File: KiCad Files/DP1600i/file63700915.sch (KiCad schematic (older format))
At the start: 22 parts, among them J1 DB25_Male, J11 Conn_01x05, J12 Conn_01x05, J13 Conn_01x05, J14 Conn_01x05, J15 Conn_01x05, J16 Conn_01x05, J17 Conn_01x05, J18 Conn_01x05, J19 Conn_01x23, J20 Conn_01x23, J21 Conn_01x17, J22 Conn_01x17, J23 Conn_01x17, J24 Conn_01x10, J25 Conn_01x10, J26 Conn_01x09, J27 Conn_01x09, J28 Conn_01x01, J29 Conn_01x02, J30 Conn_01x03, J31 Conn_01x04

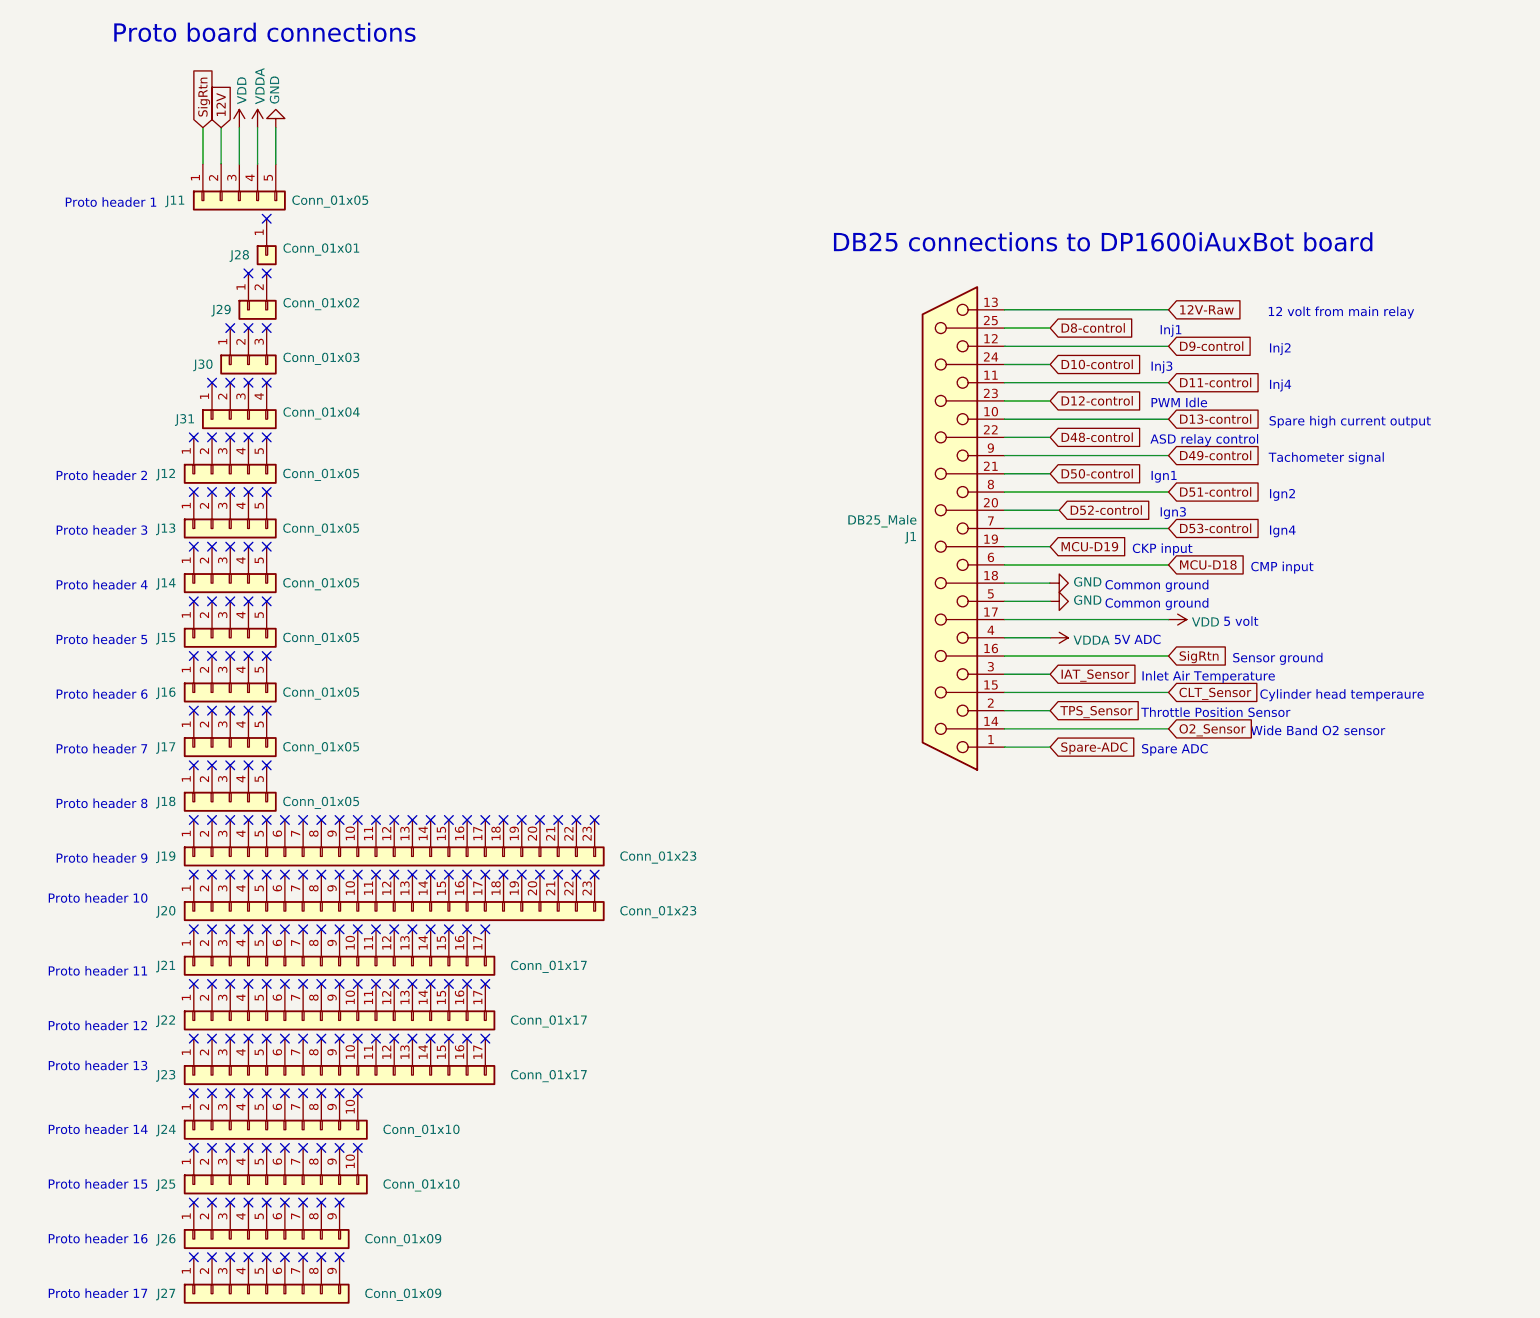
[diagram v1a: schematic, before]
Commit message: Add files via upload
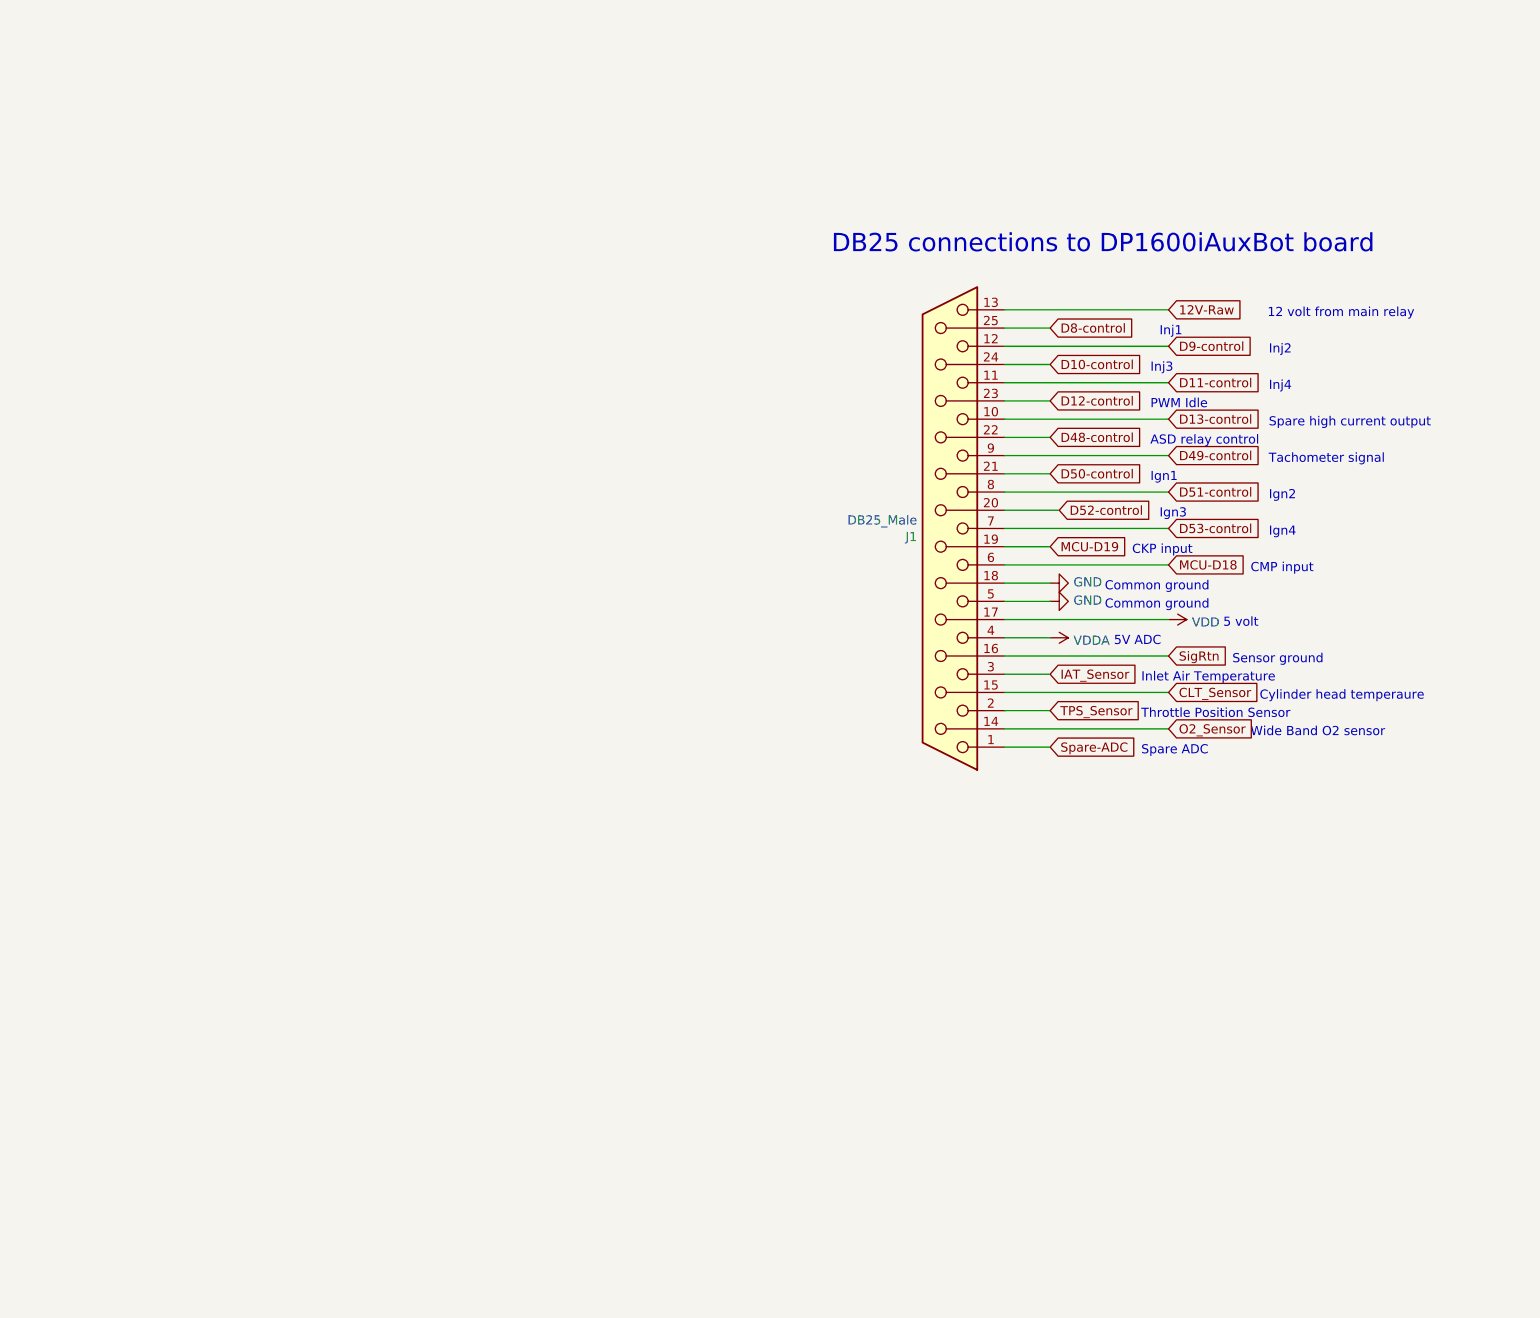
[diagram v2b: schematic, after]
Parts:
- removed J11, J12, J13, J14, J15, J16, J17, J18: Conn_01x05, Connector_PinHeader_2.54mm:PinHeader_1x05_P2.54mm_Vertical, symbol Connector_Generic:Conn_01x05
- removed J19, J20: Conn_01x23, Connector_PinHeader_2.54mm:PinHeader_1x23_P2.54mm_Vertical, symbol Connector_Generic:Conn_01x23
- removed J21, J22, J23: Conn_01x17, Connector_PinHeader_2.54mm:PinHeader_1x17_P2.54mm_Vertical, symbol Connector_Generic:Conn_01x17
- removed J24, J25: Conn_01x10, Connector_PinHeader_2.54mm:PinHeader_1x10_P2.54mm_Vertical, symbol Connector_Generic:Conn_01x10
- removed J26, J27: Conn_01x09, Connector_PinHeader_2.54mm:PinHeader_1x09_P2.54mm_Vertical, symbol Connector_Generic:Conn_01x09
- removed J28: Conn_01x01, Connector_PinHeader_2.54mm:PinHeader_1x01_P2.54mm_Vertical, symbol Connector_Generic:Conn_01x01
- removed J29: Conn_01x02, Connector_PinHeader_2.54mm:PinHeader_1x02_P2.54mm_Vertical, symbol Connector_Generic:Conn_01x02
- removed J30: Conn_01x03, Connector_PinHeader_2.54mm:PinHeader_1x03_P2.54mm_Vertical, symbol Connector_Generic:Conn_01x03
- removed J31: Conn_01x04, Connector_PinHeader_2.54mm:PinHeader_1x04_P2.54mm_Vertical, symbol Connector_Generic:Conn_01x04
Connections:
- no-connect marks 180 -> 0
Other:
- note removed: "Proto board connections\n"
- note removed: "Proto header 1"
- note removed: "Proto header 10\n\n"
- note removed: "Proto header 11\n\n"
- note removed: "Proto header 12\n\n"
- note removed: "Proto header 13\n\n\n"
- note removed: "Proto header 14\n\n\n"
- note removed: "Proto header 15\n\n\n"
- note removed: "Proto header 16\n\n\n"
- note removed: "Proto header 17\n\n\n"
- note removed: "Proto header 2"
- note removed: "Proto header 3"
- note removed: "Proto header 4"
- note removed: "Proto header 5"
- note removed: "Proto header 6"
- note removed: "Proto header 7"
- note removed: "Proto header 8"
- note removed: "Proto header 9\n"
